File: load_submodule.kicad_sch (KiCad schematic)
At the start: 8 parts, among them Q1 RFP30N06LE

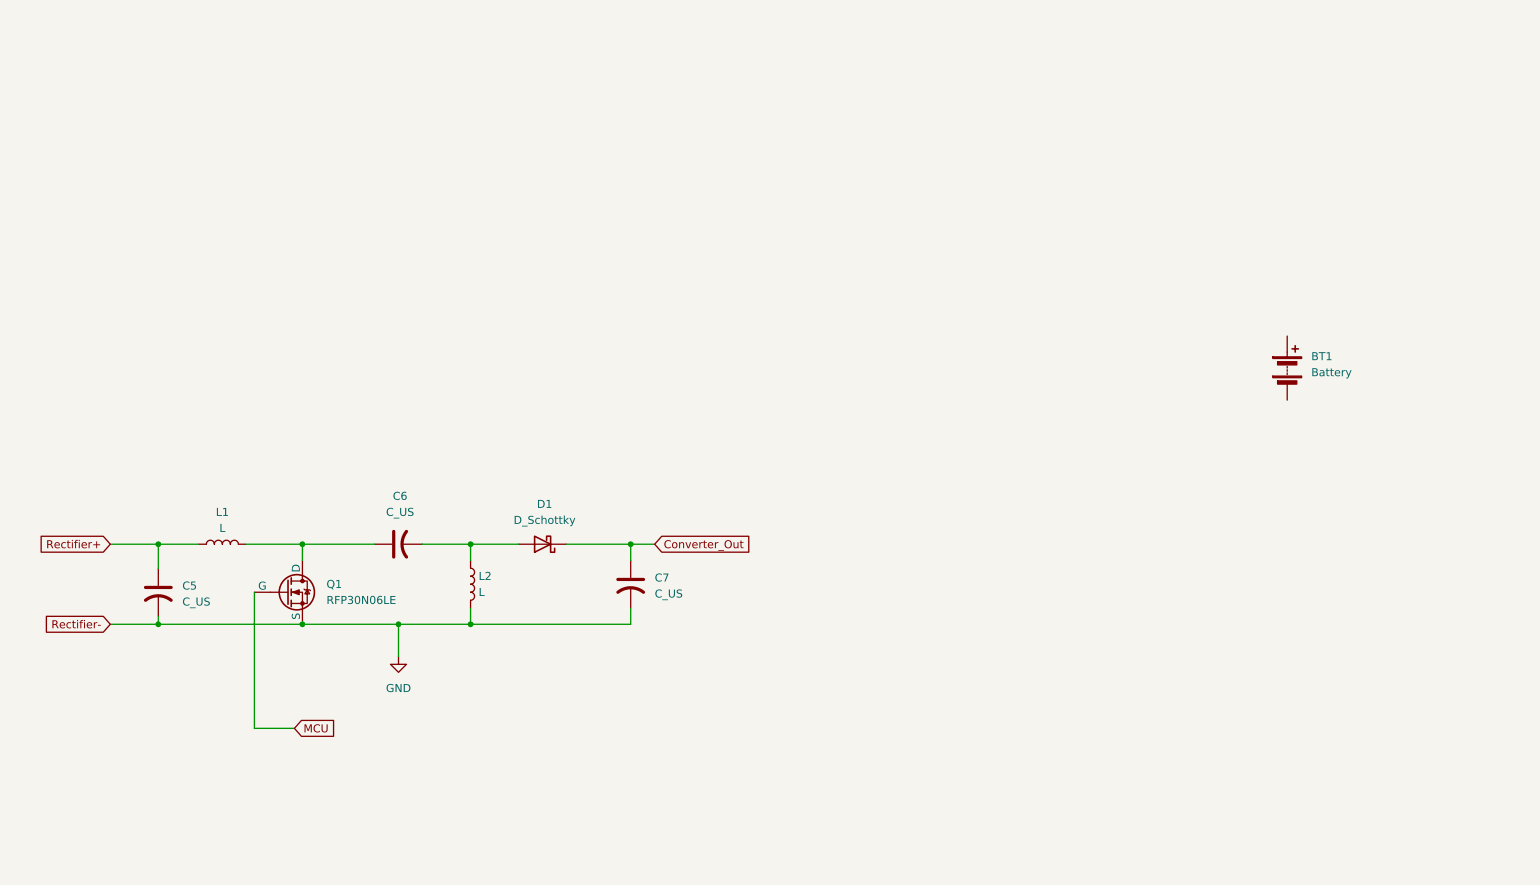
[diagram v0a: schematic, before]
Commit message: Included Shunt Values
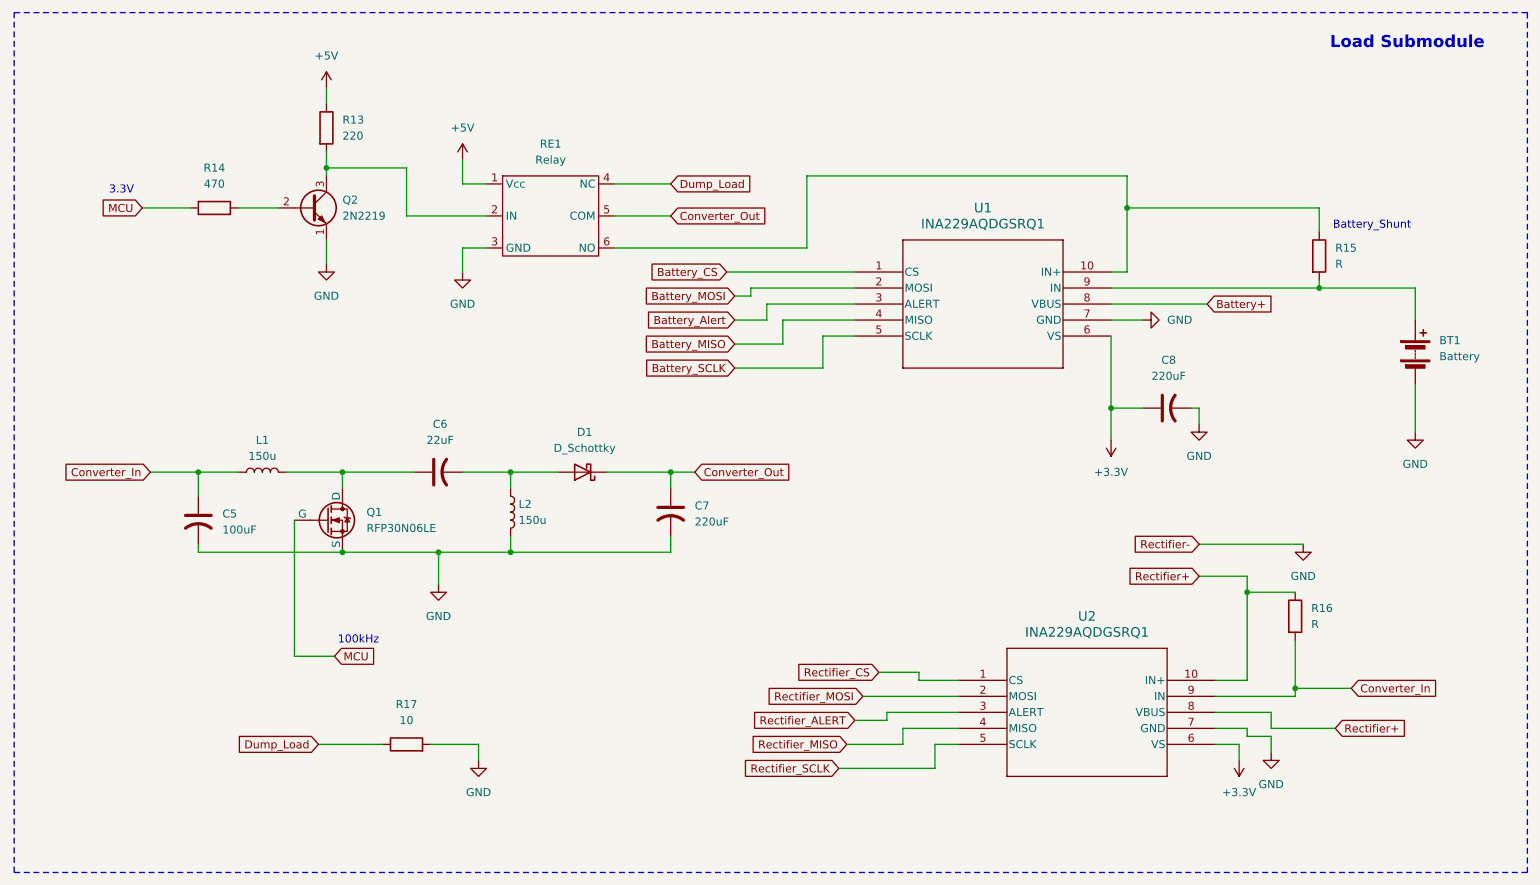
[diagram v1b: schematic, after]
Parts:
- added C8: 220uF, symbol Device:C_US
- added Q2: 2N2219, Package_TO_SOT_THT:TO-39-3, symbol Transistor_BJT:2N2219
- added R13: 220, symbol Device:R
- added R14: 470, symbol Device:R
- added R15, R16: R, symbol Device:R
- added R17: 10, symbol Device:R
- added RE1: Relay, symbol windTurbineSchemSymLib:Relay
- added U1, U2: INA229AQDGSRQ1, VSSOP10_DGS_TEX, symbol INA229:INA229AQDGSRQ1
- C5: value C_US -> 100uF
- C6: value C_US -> 22uF
- C7: value C_US -> 220uF
- L1, L2: value L -> 150u
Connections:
- net Converter_Out: now also RE1.5 (COM)
- net GND: now also BT1.2 (-), C8.2, Q2.1 (E), R17.2, RE1.3 (GND), U1.7 (GND), U2.7 (GND)
- net MCU: now also R14.1
- net Rectifier+: now also R16.1, U2.10 (IN+), U2.8 (VBUS); no longer C5.1, L1.1
- net at BT1.1 (+): now also R15.2, U1.9 (IN)
- new net: Q2.3 (C), R13.2, RE1.2 (IN)
- new net: Q2.2 (B), R14.2
- new net: R15.1, RE1.6 (NO), U1.10 (IN+)
- new net +3.3V: C8.1, U1.6 (VS), U2.6 (VS)
- new net +5V: R13.1, RE1.1 (Vcc)
- new net Battery+: U1.8 (VBUS)
- new net Battery_Alert: U1.3 (ALERT)
- new net Battery_CS: U1.1 (CS)
- new net Battery_MISO: U1.4 (MISO)
- new net Battery_MOSI: U1.2 (MOSI)
- new net Battery_SCLK: U1.5 (SCLK)
- new net Converter_In: C5.1, L1.1, R16.2, U2.9 (IN)
- new net Dump_Load: R17.1, RE1.4 (NC)
- new net Rectifier_ALERT: U2.3 (ALERT)
- new net Rectifier_CS: U2.1 (CS)
- new net Rectifier_MISO: U2.4 (MISO)
- new net Rectifier_MOSI: U2.2 (MOSI)
- new net Rectifier_SCLK: U2.5 (SCLK)
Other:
- note added: "100kHz"
- note added: "3.3V"
- note added: "Battery_Shunt"
- note added: "Load Submodule"
- moved on the sheet: BT1, C5, C6, C7, D1, L1, L2, Q1
